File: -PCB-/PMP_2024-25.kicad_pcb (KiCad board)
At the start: 2 copper layers, 60 x 110 mm, 50 parts, among them J1 5V, J2 GND, J3 OUT, J4 TEST, Q1 NPN 2N3904, Q2 NPN 2N3904, Q3 NPN MPSA42, Q4 NPN 2N3904

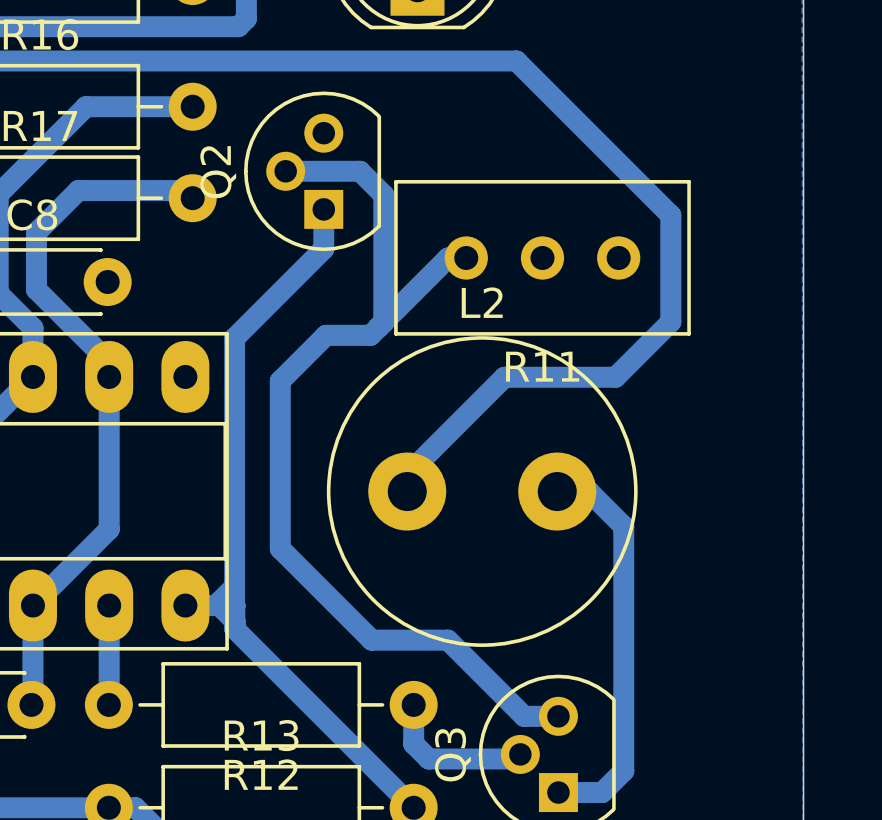
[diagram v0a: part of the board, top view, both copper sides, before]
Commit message: presentation update
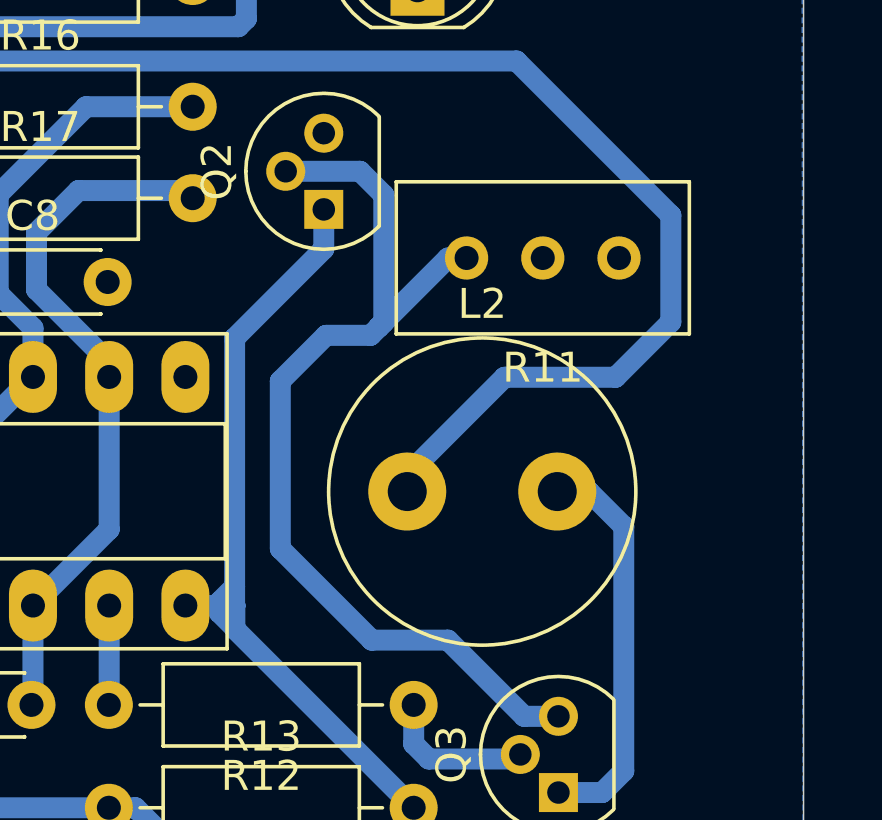
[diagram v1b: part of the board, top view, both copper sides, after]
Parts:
- moved TP1 135.7 mm to (44.8, 53.8), turned to 180 degrees
